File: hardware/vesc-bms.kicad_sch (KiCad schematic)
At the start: 1 part

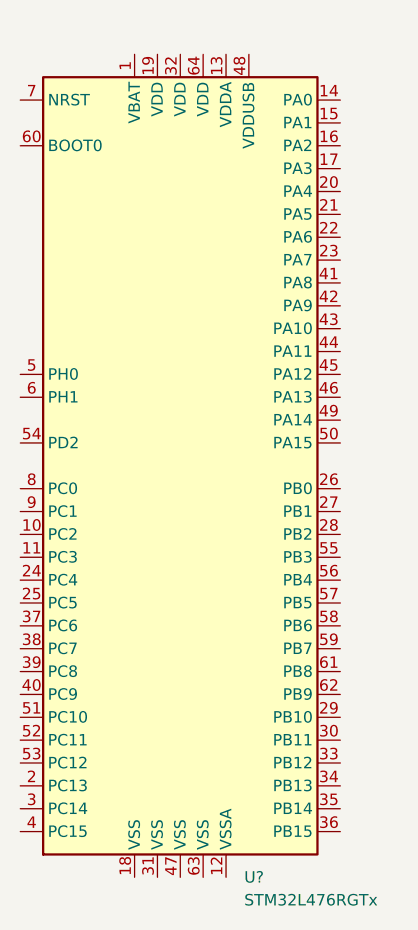
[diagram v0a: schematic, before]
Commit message: MCU schematics
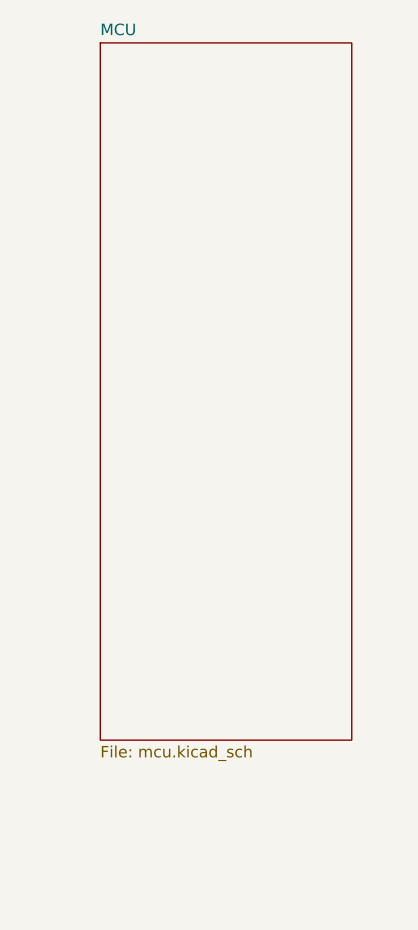
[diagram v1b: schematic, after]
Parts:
- removed U?: STM32L476RGTx, Package_QFP:LQFP-64_10x10mm_P0.5mm, symbol MCU_ST_STM32L4:STM32L476RGTx
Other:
- added sheet MCU (mcu.kicad_sch)
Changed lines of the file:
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@@
 (kicad_sch (version 20211123) (generator eeschema)
   (paper "A4")
-  (symbol (lib_id "MCU_ST_STM32L4:STM32L476RGTx") (at 143.51 95.25 0) (unit 1)
-    (in_bom yes) (on_board yes) (fields_autoplaced)
-    (property "Reference" "U?" (id 0) (at 150.6094 140.97 0)
-      (effects (font (size 1.27 1.27)) (justify left))
+  (sheet (at 134.62 48.26) (size 27.94 77.47) (fields_autoplaced)
+    (stroke (width 0.1524) (type solid) (color 0 0 0 0))
+    (fill (color 0 0 0 0.0000))
+    (property "Sheet name" "MCU" (id 0) (at 134.62 47.5484 0)
+      (effects (font (size 1.27 1.27)) (justify left bottom))
     )
-    (property "Value" "STM32L476RGTx" (id 1) (at 150.6094 143.51 0)
-      (effects (font (size 1.27 1.27)) (justify left))
+    (property "Sheet file" "mcu.kicad_sch" (id 1) (at 134.62 126.3146 0)
+      (effects (font (size 1.27 1.27)) (justify left top))
     )
-    (property "Footprint" "Package_QFP:LQFP-64_10x10mm_P0.5mm" (id 2) (at 128.27 138.43 0)
-      (effects (font (size 1.27 1.27)) (justify right) hide)
-    )
-    (property "Datasheet" "http://www.st.com/st-web-ui/static/active/en/resource/technical/document/datasheet/DM00108832.pdf" (id 3) (at 143.51 95.25 0)
-      (effects (font (size 1.27 1.27)) hide)
-    )
-    (pin "1")
-    (pin "10")
-    (pin "11")
-    (pin "12")
-    (pin "13")
-    (pin "14")
-    (pin "15")
-    (pin "16")
-    (pin "17")
-    (pin "18")
-    (pin "19")
-    (pin "2")
-    (pin "20")
-    (pin "21")
-    (pin "22")
-    (pin "23")
-    (pin "24")
-    (pin "25")
-    (pin "26")
-    (pin "27")
-    (pin "28")
-    (pin "29")
-    (pin "3")
-    (pin "30")
-    (pin "31")
-    (pin "32")
-    (pin "33")
-    (pin "34")
-    (pin "35")
-    (pin "36")
-    (pin "37")
-    (pin "38")
-    (pin "39")
-    (pin "4")
-    (pin "40")
-    (pin "41")
-    (pin "42")
-    (pin "43")
-    (pin "44")
-    (pin "45")
-    (pin "46")
-    (pin "47")
-    (pin "48")
-    (pin "49")
-    (pin "5")
-    (pin "50")
-    (pin "51")
-    (pin "52")
-    (pin "53")
-    (pin "54")
-    (pin "55")
-    (pin "56")
-    (pin "57")
-    (pin "58")
-    (pin "59")
-    (pin "6")
-    (pin "60")
-    (pin "61")
-    (pin "62")
-    (pin "63")
-    (pin "64")
-    (pin "7")
-    (pin "8")
-    (pin "9")
   )
   (sheet_instances
     (path "/" (page "1"))
+    (path "/1c5935ea-6f80-435f-8ae1-741f5546f8d9" (page "2"))
   )
   (symbol_instances
-    (path "/4dc60a8b-6e80-402b-bfeb-ecf4e3929f2e"
+    (path "/1c5935ea-6f80-435f-8ae1-741f5546f8d9/04a8d2cc-4488-4f89-9bab-2ebaa2c871f9"
+      (reference "#PWR?") (unit 1) (value "GND") (footprint "")
+    )
+    (path "/1c5935ea-6f80-435f-8ae1-741f5546f8d9/0f3e1354-323d-4229-9a90-973d8aa8e10f"
+      (reference "#PWR?") (unit 1) (value "+3.3V") (footprint "")
+    )
+    (path "/1c5935ea-6f80-435f-8ae1-741f5546f8d9/330d991c-d2e7-47ad-a0dc-560b7089f626"
+      (reference "#PWR?") (unit 1) (value "+3.3V") (footprint "")
+    )
+    (path "/1c5935ea-6f80-435f-8ae1-741f5546f8d9/4995bacf-1534-43d1-a64e-fbadc52762c2"
+      (reference "#PWR?") (unit 1) (value "GND") (footprint "")
+    )
+    (path "/1c5935ea-6f80-435f-8ae1-741f5546f8d9/5790de93-f476-480c-8300-d97bb5ef83c9"
+      (reference "#PWR?") (unit 1) (value "GND") (footprint "")
+    )
+    (path "/1c5935ea-6f80-435f-8ae1-741f5546f8d9/5a3a09a7-6ac2-4390-b78c-2d4cfc84b18e"
+      (reference "#PWR?") (unit 1) (value "+3.3V") (footprint "")
+    )
+    (path "/1c5935ea-6f80-435f-8ae1-741f5546f8d9/78249a6d-7015-42c7-a31b-2e64611e12a2"
+      (reference "#PWR?") (unit 1) (value "GND") (footprint "")
+    )
+    (path "/1c5935ea-6f80-435f-8ae1-741f5546f8d9/8855f663-173b-420d-a359-12239a93dd8a"
+      (reference "#PWR?") (unit 1) (value "GND") (footprint "")
+    )
+    (path "/1c5935ea-6f80-435f-8ae1-741f5546f8d9/a541c024-5390-4ab8-93c8-694086fd6f03"
+      (reference "#PWR?") (unit 1) (value "+3.3V") (footprint "")
+    )
+    (path "/1c5935ea-6f80-435f-8ae1-741f5546f8d9/cd5791f7-0242-4035-b190-bb6078f5bcce"
+      (reference "#PWR?") (unit 1) (value "GND") (footprint "")
+    )
+    (path "/1c5935ea-6f80-435f-8ae1-741f5546f8d9/d95b970c-bb79-477d-8f2d-262e72f77908"
+      (reference "#PWR?") (unit 1) (value "GND") (footprint "")
+    )
+    (path "/1c5935ea-6f80-435f-8ae1-741f5546f8d9/e7b82764-134f-4c86-89cb-98c649d51e66"
+      (reference "#PWR?") (unit 1) (value "+3.3V") (footprint "")
+    )
+    (path "/1c5935ea-6f80-435f-8ae1-741f5546f8d9/ee39d913-28b4-409e-b803-a8f30175ff9f"
+      (reference "#PWR?") (unit 1) (value "+3.3V") (footprint "")
+    )
+    (path "/1c5935ea-6f80-435f-8ae1-741f5546f8d9/352c82b9-b682-4d46-86ce-1bc0e3adc52b"
+      (reference "C?") (unit 1) (value "1u") (footprint "")
+    )
+    (path "/1c5935ea-6f80-435f-8ae1-741f5546f8d9/3d53b2c0-0ab8-418a-a174-d479fe6d5385"
+      (reference "C?") (unit 1) (value "DNP") (footprint "Capacitor_SMD:C_0805_2012Metric")
+    )
+    (path "/1c5935ea-6f80-435f-8ae1-741f5546f8d9/582a367b-1112-4363-ad61-1bcc6e36146a"
+      (reference "C?") (unit 1) (value "100n") (footprint "Capacitor_SMD:C_0805_2012Metric")
+    )
+    (path "/1c5935ea-6f80-435f-8ae1-741f5546f8d9/6f2eed42-07e8-4208-97fd-0348bccca920"
+      (reference "C?") (unit 1) (value "100n") (footprint "")
+    )
+    (path "/1c5935ea-6f80-435f-8ae1-741f5546f8d9/7f324268-9f73-48c6-9202-6dfc802557cb"
+      (reference "C?") (unit 1) (value "DNP") (footprint "Capacitor_SMD:C_0805_2012Metric")
+    )
+    (path "/1c5935ea-6f80-435f-8ae1-741f5546f8d9/9e5dfc52-7ea2-4b6c-a9ad-4488a2b290b8"
+      (reference "C?") (unit 1) (value "100n") (footprint "")
+    )
+    (path "/1c5935ea-6f80-435f-8ae1-741f5546f8d9/a043eb2a-f7b6-4ccf-a1ff-2a14a6a2a866"
+      (reference "C?") (unit 1) (value "100n") (footprint "")
+    )
+    (path "/1c5935ea-6f80-435f-8ae1-741f5546f8d9/aac7eb03-ea6f-4bcc-bd5c-02c1a2a2e655"
+      (reference "C?") (unit 1) (value "10n") (footprint "")
+    )
+    (path "/1c5935ea-6f80-435f-8ae1-741f5546f8d9/bcc35541-7440-436b-ab2e-34d9442052d6"
+      (reference "C?") (unit 1) (value "4.7u") (footprint "")
+    )
+    (path "/1c5935ea-6f80-435f-8ae1-741f5546f8d9/fcf69119-ebcf-4353-9d24-d44f2add92c4"
+      (reference "C?") (unit 1) (value "100n") (footprint "Capacitor_SMD:C_0805_2012Metric")
+    )
+    (path "/1c5935ea-6f80-435f-8ae1-741f5546f8d9/b6cbb8ea-1784-4059-9a07-19b7c70fa644"
+      (reference "J?") (unit 1) (value "Conn_ARM_JTAG_SWD_10") (footprint "")
+    )
+    (path "/1c5935ea-6f80-435f-8ae1-741f5546f8d9/21b9b2b5-ff97-447a-a56e-396f0ea09701"
+      (reference "R?") (unit 1) (value "DNP") (footprint "Resistor_SMD:R_0805_2012Metric")
+    )
+    (path "/1c5935ea-6f80-435f-8ae1-741f5546f8d9/3a456d76-fae8-41f6-8005-597506331c4a"
+      (reference "R?") (unit 1) (value "10k") (footprint "Resistor_SMD:R_0805_2012Metric")
+    )
+    (path "/1c5935ea-6f80-435f-8ae1-741f5546f8d9/4d538473-c25c-4a8d-999f-ecd2ffd9b70a"
+      (reference "SW?") (unit 1) (value "SW_Push") (footprint "Button_Switch_SMD:SW_SPST_B3S-1000")
+    )
+    (path "/1c5935ea-6f80-435f-8ae1-741f5546f8d9/fd1a8cd8-06e9-4d52-af0e-ed2b061904eb"
+      (reference "SW?") (unit 1) (value "SW_Push") (footprint "Button_Switch_SMD:SW_SPST_B3S-1000")
+    )
+    (path "/1c5935ea-6f80-435f-8ae1-741f5546f8d9/cfe202db-7a07-41ea-849b-c0da94eb6992"
       (reference "U?") (unit 1) (value "STM32L476RGTx") (footprint "Package_QFP:LQFP-64_10x10mm_P0.5mm")
     )
+    (path "/1c5935ea-6f80-435f-8ae1-741f5546f8d9/0827f1d0-8e1d-46d4-92fd-80f7ab36b847"
+      (reference "Y?") (unit 1) (value "DNP") (footprint "Crystal:Crystal_SMD_3225-4Pin_3.2x2.5mm")
+    )
   )
